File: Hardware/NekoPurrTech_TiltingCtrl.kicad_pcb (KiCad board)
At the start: 2 copper layers, 15.3 x 20 mm, 32 parts, among them IC1 TPS70933DRVR, IC2 TB67H450FNG, IC3 TPS70933DRVR, J1 Power_IN, J2 FMU_PWM, J3 Motor, U1 STM32F030F4Px

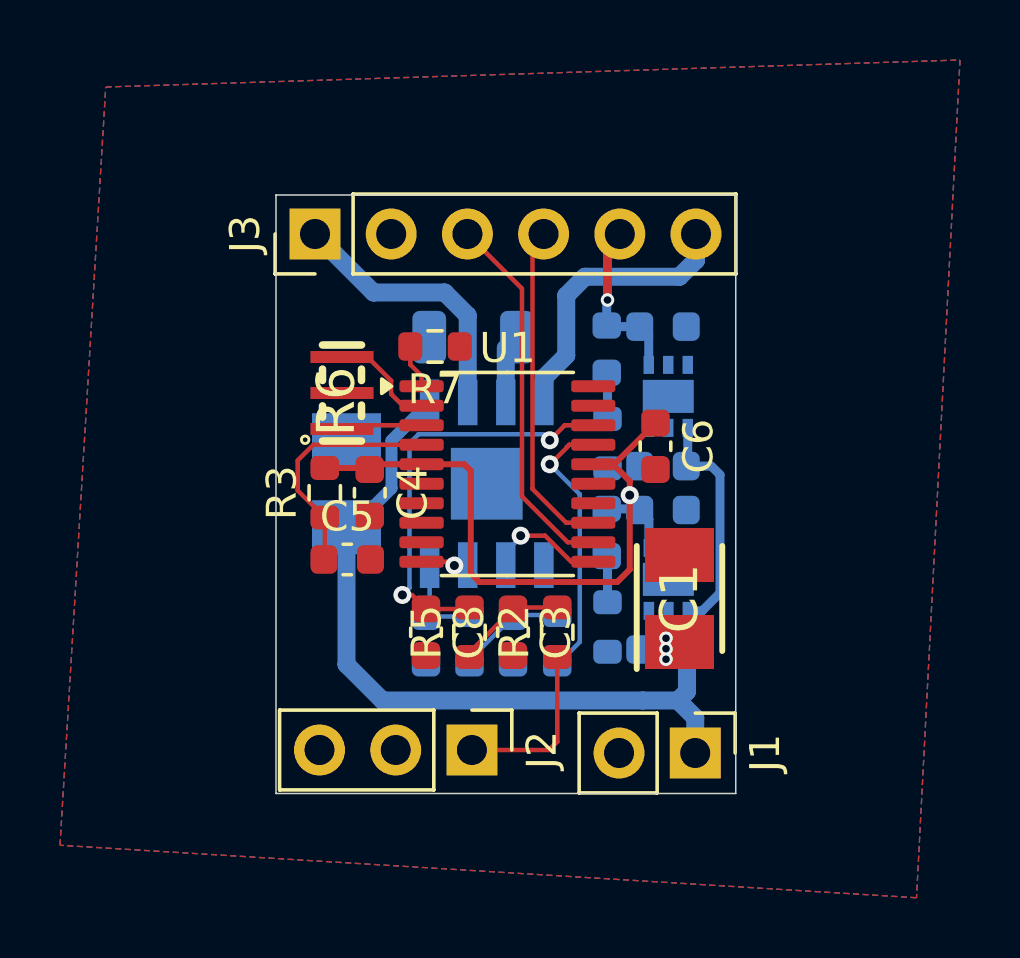
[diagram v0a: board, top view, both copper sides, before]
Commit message: Finished Hardware
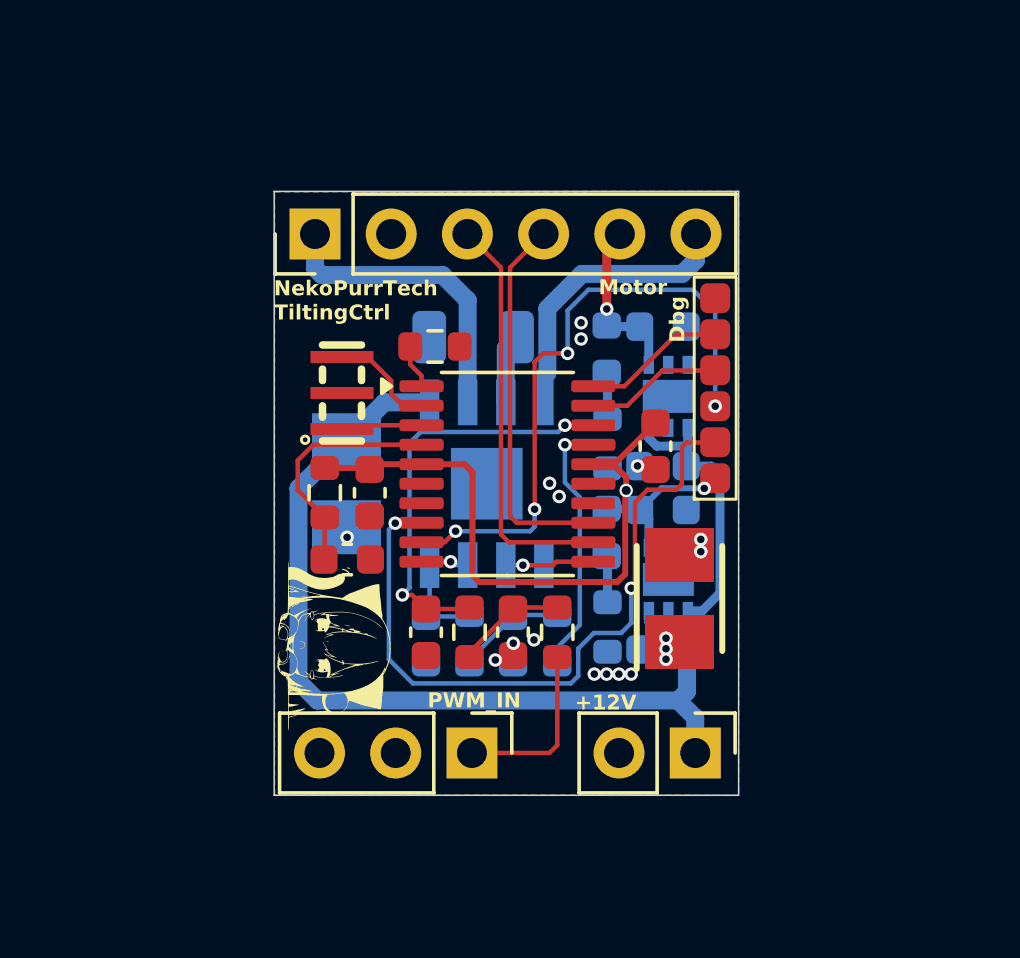
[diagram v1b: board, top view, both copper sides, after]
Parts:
- added ?: , SamacSys_Parts:nya_mini, F.Cu at (86.9, 70.0)
- added J4: Dbg_Port, SamacSys_Parts:Dbg_Port, F.Cu at (99.7, 61.4)
- moved J2 0.10 mm to (91.6, 73.6)
- turned C12 to -90 degrees
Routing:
- net /Dbg_TX: track 0.00 -> 23.4 mm, vias 0 -> 2
- net /Dbg_RX: track 0.00 -> 21.0 mm, vias 0 -> 4
- net VCC: track 38.6 -> 46.6 mm
- net /SWCLK: track 0.00 -> 4.55 mm
- net /SWDIO: track 0.00 -> 4.32 mm
- net +3.3V_MCU: track 24.2 -> 27.2 mm, vias 1 -> 2
- net /ENC_B: track 11.1 -> 12.7 mm
- net /ENC_A: track 12.5 -> 13.7 mm
- net /IN2: track 3.97 -> 2.97 mm
- net /Motor+: track 9.11 -> 10.1 mm
- net GND: track 0.00 -> 0.72 mm, vias 0 -> 15
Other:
- board size 15.3 x 20 mm -> 15.5 x 20.1 mm
- board text added: "+12V"
- board text added: "Dbg"
- board text added: "Motor"
- board text added: "NekoPurrTech TiltingCtrl"
- board text added: "PWM_IN"
